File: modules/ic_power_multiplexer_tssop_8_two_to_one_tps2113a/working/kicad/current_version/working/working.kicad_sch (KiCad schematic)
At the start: 3 parts, among them IC1 itssp8mpptps2113

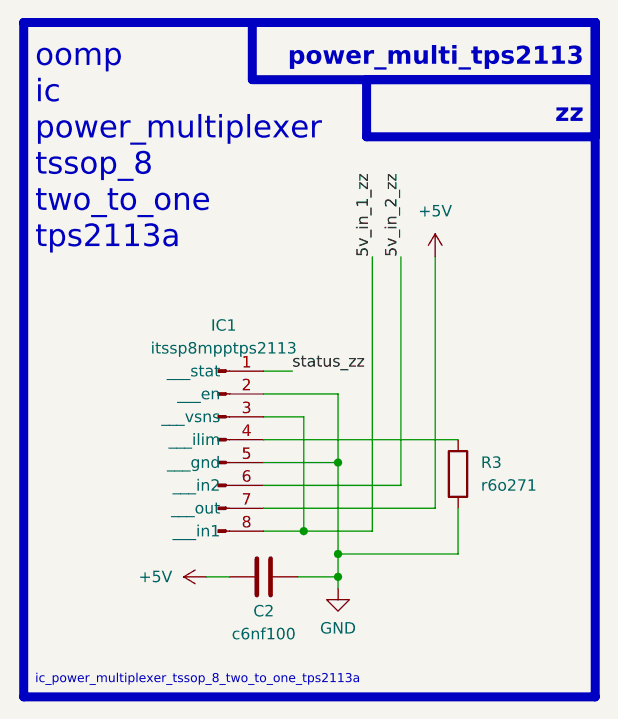
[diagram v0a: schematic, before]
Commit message: some works
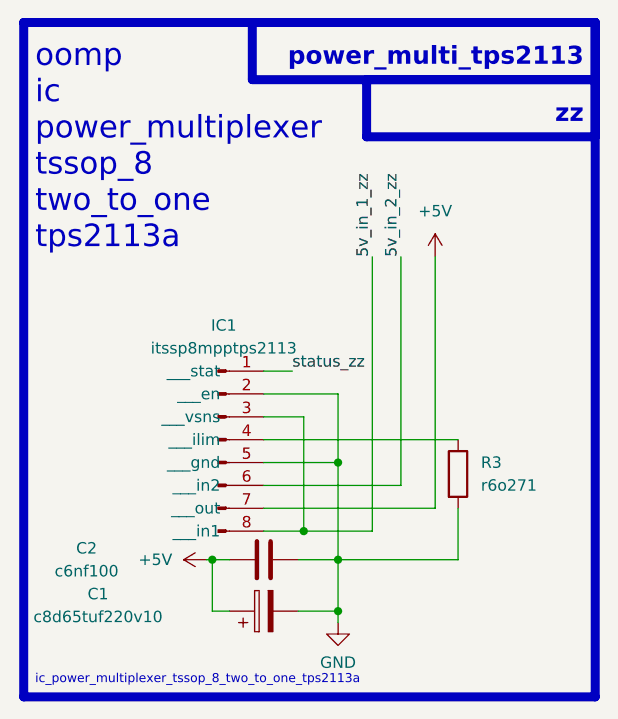
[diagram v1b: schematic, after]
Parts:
- added C1: c8d65tuf220v10, oomlout_oomp_part_footprints:c8d65tuf220v10_electronic_capacitor_8_mm_diameter_6_5_mm_tall_electrolytic_220_micro_farad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, symbol oomlout_oomp_part_symbols:c8d65tuf220v10_electronic_capacitor_8_mm_diameter_6_5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
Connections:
- net +5V: now also C1.1
- net GND: now also C1.2
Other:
- moved on the sheet: C2
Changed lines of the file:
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@@
 (kicad_sch (version 20230121) (generator eeschema)
   (paper "A5")
-  (junction (at 108.585 97.155) (diameter 0) (color 0 0 0 0)
+  (junction (at 108.585 95.25) (diameter 0) (color 0 0 0 0)
   )
   (junction (at 108.585 84.455) (diameter 0) (color 0 0 0 0)
   )
-  (junction (at 108.585 94.615) (diameter 0) (color 0 0 0 0)
+  (junction (at 108.585 100.965) (diameter 0) (color 0 0 0 0)
   )
   (junction (at 104.775 92.075) (diameter 0) (color 0 0 0 0)
   )
+  (junction (at 94.615 95.25) (diameter 0) (color 0 0 0 0)
+  )
   (wire (pts (xy 100.33 74.295) (xy 103.505 74.295))
     (stroke (width 0) (type default))
@@
     (stroke (width 0) (type default))
   )
-  (wire (pts (xy 108.585 97.155) (xy 108.585 98.425))
-    (stroke (width 0) (type default))
-  )
-  (wire (pts (xy 121.92 94.615) (xy 121.92 89.535))
+  (wire (pts (xy 108.585 100.965) (xy 108.585 102.235))
+    (stroke (width 0) (type default))
+  )
+  (wire (pts (xy 121.92 89.535) (xy 121.92 95.25))
+    (stroke (width 0) (type default))
+  )
+  (wire (pts (xy 94.615 100.965) (xy 94.615 95.25))
+    (stroke (width 0) (type default))
+  )
+  (wire (pts (xy 96.52 100.965) (xy 94.615 100.965))
     (stroke (width 0) (type default))
   )
@@
     (stroke (width 0) (type default))
   )
-  (wire (pts (xy 104.14 97.155) (xy 108.585 97.155))
-    (stroke (width 0) (type default))
-  )
   (wire (pts (xy 100.33 81.915) (xy 121.92 81.915))
     (stroke (width 0) (type default))
   )
-  (wire (pts (xy 108.585 94.615) (xy 108.585 97.155))
-    (stroke (width 0) (type default))
-  )
   (wire (pts (xy 108.585 84.455) (xy 100.33 84.455))
     (stroke (width 0) (type default))
   )
+  (wire (pts (xy 104.14 100.965) (xy 108.585 100.965))
+    (stroke (width 0) (type default))
+  )
   (wire (pts (xy 115.57 86.995) (xy 100.33 86.995))
     (stroke (width 0) (type default))
   )
+  (wire (pts (xy 104.14 95.25) (xy 108.585 95.25))
+    (stroke (width 0) (type default))
+  )
   (wire (pts (xy 100.33 76.835) (xy 108.585 76.835))
     (stroke (width 0) (type default))
   )
-  (wire (pts (xy 108.585 94.615) (xy 121.92 94.615))
-    (stroke (width 0) (type default))
-  )
-  (wire (pts (xy 93.98 97.155) (xy 96.52 97.155))
+  (wire (pts (xy 93.98 95.25) (xy 94.615 95.25))
     (stroke (width 0) (type default))
   )
@@
     (stroke (width 0) (type default))
   )
-  (wire (pts (xy 108.585 94.615) (xy 108.585 84.455))
+  (wire (pts (xy 108.585 84.455) (xy 108.585 95.25))
+    (stroke (width 0) (type default))
+  )
+  (wire (pts (xy 94.615 95.25) (xy 96.52 95.25))
+    (stroke (width 0) (type default))
+  )
+  (wire (pts (xy 121.92 95.25) (xy 108.585 95.25))
     (stroke (width 0) (type default))
   )
   (wire (pts (xy 100.33 92.075) (xy 104.775 92.075))
+    (stroke (width 0) (type default))
+  )
+  (wire (pts (xy 108.585 95.25) (xy 108.585 100.965))
     (stroke (width 0) (type default))
   )
@@
     (effects (font (size 1.27 1.27)) (justify left bottom))
   )
-  (symbol (lib_id "oomlout_oomp_part_symbols:c6nf100_electronic_capacitor_0603_100_nano_farad") (at 100.33 97.155 90) (unit 1)
+  (symbol (lib_id "oomlout_oomp_part_symbols:c6nf100_electronic_capacitor_0603_100_nano_farad") (at 100.33 95.25 90) (unit 1)
     (in_bom yes) (on_board yes) (dnp no)
-    (property "Reference" "C2" (at 100.33 100.965 90)
-      (effects (font (size 1.27 1.27)))
-    )
-    (property "Value" "c6nf100" (at 100.33 103.505 90)
-      (effects (font (size 1.27 1.27)))
-    )
-    (property "Footprint" "oomlout_oomp_part_footprints:c6nf100_electronic_capacitor_0603_100_nano_farad" (at 104.14 96.1898 0)
-      (effects (font (size 1.27 1.27)) hide)
-    )
-    (property "Datasheet" "https://github.com/oomlout/oomlout_oomp_v3/parts/electronic_capacitor_0603_100_nano_farad/datasheet.pdf" (at 100.33 97.155 0)
+    (property "Reference" "C2" (at 80.645 93.98 90)
+      (effects (font (size 1.27 1.27)))
+    )
+    (property "Value" "c6nf100" (at 80.645 96.52 90)
+      (effects (font (size 1.27 1.27)))
+    )
+    (property "Footprint" "oomlout_oomp_part_footprints:c6nf100_electronic_capacitor_0603_100_nano_farad" (at 104.14 94.2848 0)
+      (effects (font (size 1.27 1.27)) hide)
+    )
+    (property "Datasheet" "https://github.com/oomlout/oomlout_oomp_v3/parts/electronic_capacitor_0603_100_nano_farad/datasheet.pdf" (at 100.33 95.25 0)
       (effects (font (size 1.27 1.27)) hide)
     )
@@
     )
   )
-  (symbol (lib_id "power:GND") (at 108.585 98.425 0) (unit 1)
+  (symbol (lib_id "oomlout_oomp_part_symbols:c8d65tuf220v10_electronic_capacitor_8_mm_diameter_6_5_mm_tall_electrolytic_220_micro_farad_10_volt") (at 100.33 100.965 90) (unit 1)
+    (in_bom yes) (on_board yes) (dnp no)
+    (property "Reference" "C1" (at 81.915 99.06 90)
+      (effects (font (size 1.27 1.27)))
+    )
+    (property "Value" "c8d65tuf220v10" (at 81.915 101.6 90)
+      (effects (font (size 1.27 1.27)))
+    )
+    (property "Footprint" "oomlout_oomp_part_footprints:c8d65tuf220v10_electronic_capacitor_8_mm_diameter_6_5_mm_tall_electrolytic_220_micro_farad_10_volt" (at 104.14 99.9998 0)
+      (effects (font (size 1.27 1.27)) hide)
+    )
+    (property "Datasheet" "https://github.com/oomlout/oomlout_oomp_v3/parts/electronic_capacitor_8_mm_diameter_6_5_mm_tall_electrolytic_220_micro_farad_10_volt/datasheet.pdf" (at 100.33 100.965 0)
+      (effects (font (size 1.27 1.27)) hide)
+    )
+    (pin "1")
+    (pin "2")
+    (instances
+      (project "working"
+        (path "/c9993764-076f-44f6-bf4c-6b69ce17c9e4"
+          (reference "C1") (unit 1)
+        )
+      )
+    )
+  )
+  (symbol (lib_id "power:GND") (at 108.585 102.235 0) (unit 1)
     (in_bom yes) (on_board yes) (dnp no) (fields_autoplaced)
-    (property "Reference" "#PWR05" (at 108.585 104.775 0)
-      (effects (font (size 1.27 1.27)) hide)
-    )
-    (property "Value" "GND" (at 108.585 102.87 0)
-      (effects (font (size 1.27 1.27)))
-    )
-    (property "Footprint" "" (at 108.585 98.425 0)
-      (effects (font (size 1.27 1.27)) hide)
-    )
-    (property "Datasheet" "" (at 108.585 98.425 0)
+    (property "Reference" "#PWR05" (at 108.585 108.585 0)
+      (effects (font (size 1.27 1.27)) hide)
+    )
+    (property "Value" "GND" (at 108.585 106.68 0)
+      (effects (font (size 1.27 1.27)))
+    )
+    (property "Footprint" "" (at 108.585 102.235 0)
+      (effects (font (size 1.27 1.27)) hide)
+    )
+    (property "Datasheet" "" (at 108.585 102.235 0)
       (effects (font (size 1.27 1.27)) hide)
     )
@@
     )
   )
-  (symbol (lib_id "power:+5V") (at 93.98 97.155 90) (unit 1)
+  (symbol (lib_id "power:+5V") (at 93.98 95.25 90) (unit 1)
     (in_bom yes) (on_board yes) (dnp no) (fields_autoplaced)
-    (property "Reference" "#PWR01" (at 97.79 97.155 0)
-      (effects (font (size 1.27 1.27)) hide)
-    )
-    (property "Value" "+5V" (at 90.17 97.155 90)
+    (property "Reference" "#PWR01" (at 97.79 95.25 0)
+      (effects (font (size 1.27 1.27)) hide)
+    )
+    (property "Value" "+5V" (at 90.17 95.25 90)
       (effects (font (size 1.27 1.27)) (justify left))
     )
-    (property "Footprint" "" (at 93.98 97.155 0)
-      (effects (font (size 1.27 1.27)) hide)
-    )
-    (property "Datasheet" "" (at 93.98 97.155 0)
-      (effects (font (size 1.27 1.27)) hide)
-    )
+    (property "Footprint" "" (at 93.98 95.25 0)
+      (effects (font (size 1.27 1.27)) hide)
+    )
+    (property "Datasheet" "" (at 93.98 95.25 0)
+      (effects (font (size 1.27 1.27)) hide)
+    )
